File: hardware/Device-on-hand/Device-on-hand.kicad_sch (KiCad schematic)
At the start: 6 parts, among them J1 Conn_01x08, J2 Conn_01x08, J3 Conn_01x02, U1 SparkFun_SEN-14480_H3LIS331DL, U2 ESP32-DEVKIT-V1

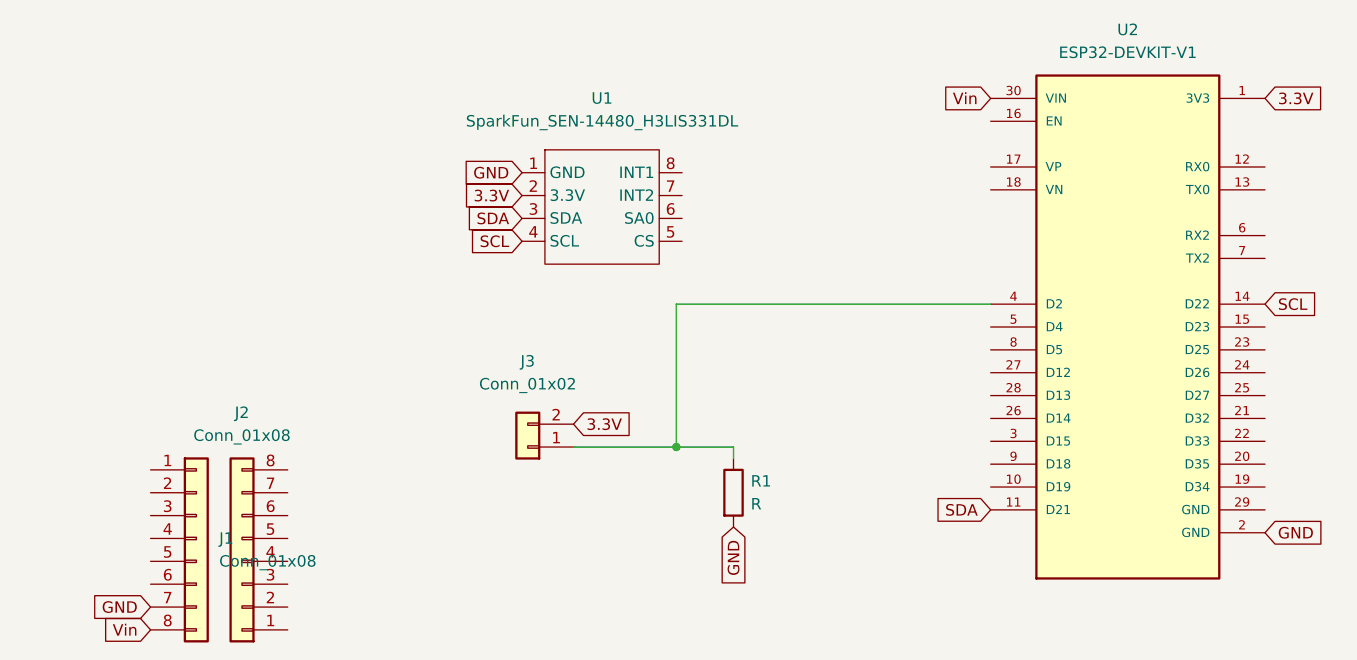
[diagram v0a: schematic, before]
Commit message: update
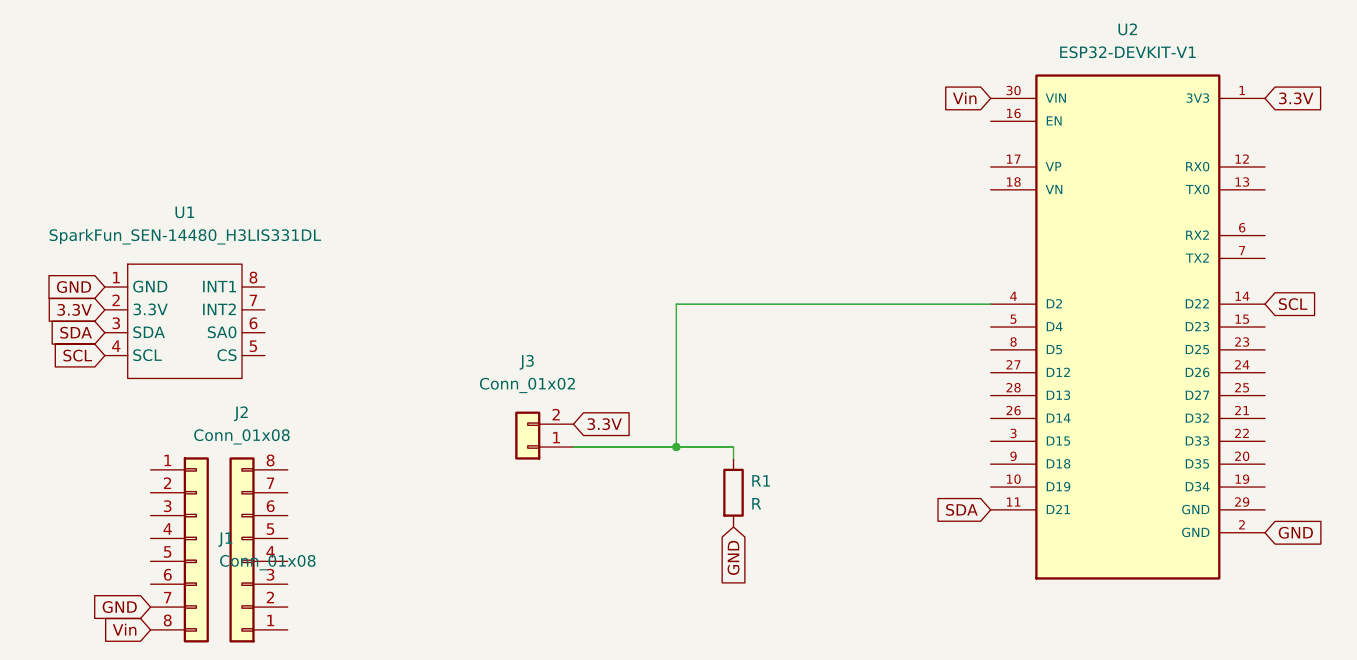
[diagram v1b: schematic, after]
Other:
- moved on the sheet: U1
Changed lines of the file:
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@@
     )
   )
-  (global_label "SCL" (shape input) (at 142.875 84.455 180) (fields_autoplaced)
+  (global_label "SCL" (shape input) (at 96.52 97.155 180) (fields_autoplaced)
     (effects (font (size 1.27 1.27)) (justify right))
-    (property "Intersheet References" "${INTERSHEET_REFS}" (id 0) (at 136.9543 84.3756 0)
+    (property "Intersheet References" "${INTERSHEET_REFS}" (id 0) (at 90.5993 97.0756 0)
       (effects (font (size 1.27 1.27)) (justify right) hide)
     )
@@
     )
   )
-  (global_label "GND" (shape input) (at 142.875 76.835 180) (fields_autoplaced)
+  (global_label "GND" (shape input) (at 96.52 89.535 180) (fields_autoplaced)
     (effects (font (size 1.27 1.27)) (justify right))
-    (property "Intersheet References" "${INTERSHEET_REFS}" (id 0) (at 136.5914 76.7556 0)
+    (property "Intersheet References" "${INTERSHEET_REFS}" (id 0) (at 90.2364 89.4556 0)
       (effects (font (size 1.27 1.27)) (justify right) hide)
     )
@@
     )
   )
-  (global_label "3.3V" (shape input) (at 142.875 79.375 180) (fields_autoplaced)
+  (global_label "3.3V" (shape input) (at 96.52 92.075 180) (fields_autoplaced)
     (effects (font (size 1.27 1.27)) (justify right))
-    (property "Intersheet References" "${INTERSHEET_REFS}" (id 0) (at 136.3495 79.2956 0)
+    (property "Intersheet References" "${INTERSHEET_REFS}" (id 0) (at 89.9945 91.9956 0)
       (effects (font (size 1.27 1.27)) (justify right) hide)
     )
   )
-  (global_label "SDA" (shape input) (at 142.875 81.915 180) (fields_autoplaced)
+  (global_label "SDA" (shape input) (at 96.52 94.615 180) (fields_autoplaced)
     (effects (font (size 1.27 1.27)) (justify right))
-    (property "Intersheet References" "${INTERSHEET_REFS}" (id 0) (at 136.8938 81.8356 0)
+    (property "Intersheet References" "${INTERSHEET_REFS}" (id 0) (at 90.5388 94.5356 0)
       (effects (font (size 1.27 1.27)) (justify right) hide)
     )
@@
     (pin "2")
   )
-  (symbol (lib_id "H3LIS331DL:SparkFun_SEN-14480_H3LIS331DL") (at 151.765 80.645 0) (unit 1)
+  (symbol (lib_id "H3LIS331DL:SparkFun_SEN-14480_H3LIS331DL") (at 105.41 93.345 0) (unit 1)
     (in_bom yes) (on_board yes) (fields_autoplaced)
-    (property "Reference" "U1" (id 0) (at 151.765 68.58 0))
-    (property "Value" "SparkFun_SEN-14480_H3LIS331DL" (id 1) (at 151.765 71.12 0))
-    (property "Footprint" "SparkFun_Tri_Axis_Accel_Breakout-H3LIS331DL:SparkFun_Tri_Axis_Accel_Breakout-H3LIS331DL" (id 2) (at 151.765 80.645 0)
+    (property "Reference" "U1" (id 0) (at 105.41 81.28 0))
+    (property "Value" "SparkFun_SEN-14480_H3LIS331DL" (id 1) (at 105.41 83.82 0))
+    (property "Footprint" "SparkFun_Tri_Axis_Accel_Breakout-H3LIS331DL:SparkFun_Tri_Axis_Accel_Breakout-H3LIS331DL" (id 2) (at 105.41 93.345 0)
       (effects (font (size 1.27 1.27)) hide)
     )
-    (property "Datasheet" "" (id 3) (at 151.765 80.645 0)
+    (property "Datasheet" "" (id 3) (at 105.41 93.345 0)
       (effects (font (size 1.27 1.27)) hide)
     )

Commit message: final commit i hope
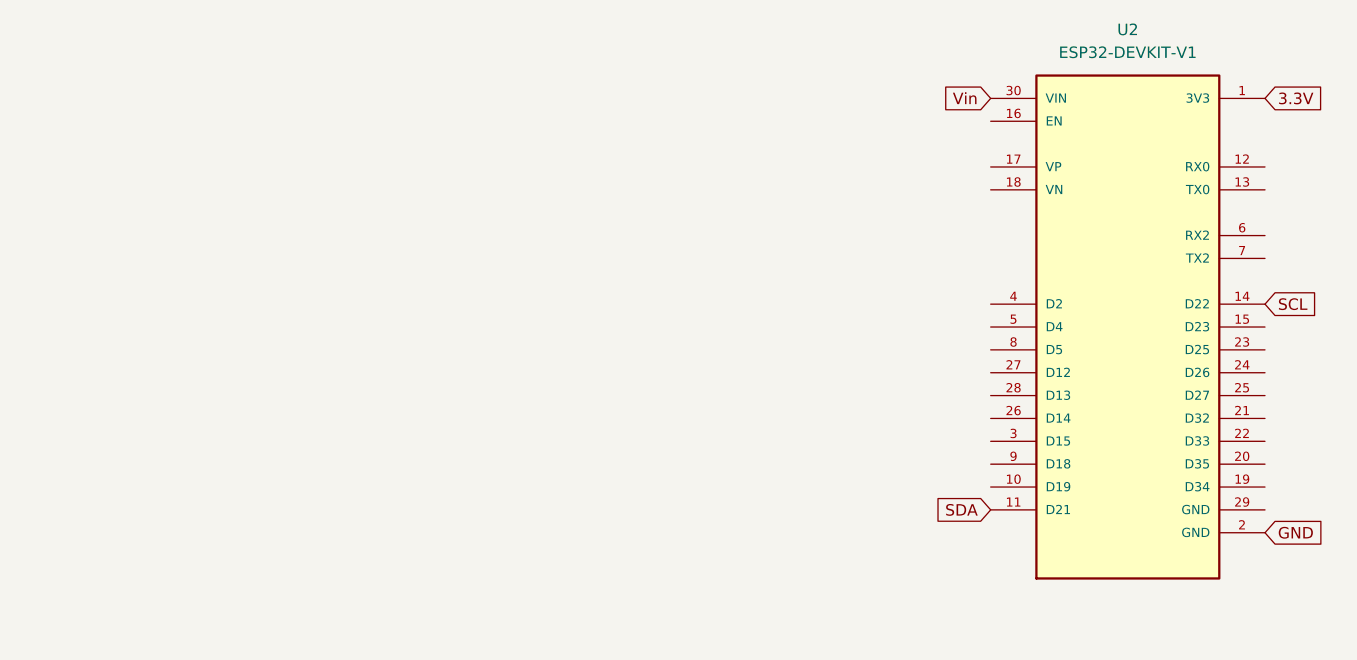
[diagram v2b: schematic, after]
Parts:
- removed J1, J2: Conn_01x08, Connector_PinSocket_2.54mm:PinSocket_1x08_P2.54mm_Vertical, symbol Connector_Generic:Conn_01x08
- removed J3: Conn_01x02, TerminalBlock_Phoenix:TerminalBlock_Phoenix_MKDS-1,5-2-5.08_1x02_P5.08mm_Horizontal, symbol Connector_Generic:Conn_01x02
- removed R1: R, Resistor_THT:R_Axial_DIN0207_L6.3mm_D2.5mm_P10.16mm_Horizontal, symbol Device:R
- removed U1: SparkFun_SEN-14480_H3LIS331DL, SparkFun_Tri_Axis_Accel_Breakout-H3LIS331DL:SparkFun_Tri_Axis_Accel_Breakout-H3LIS331DL, symbol H3LIS331DL:SparkFun_SEN-14480_H3LIS331DL
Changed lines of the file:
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@@
 (kicad_sch (version 20211123) (generator eeschema)
   (paper "A4")
-  (junction (at 160.02 107.315) (diameter 0) (color 0 0 0 0)
-  )
-  (wire (pts (xy 148.59 107.315) (xy 160.02 107.315))
-    (stroke (width 0) (type default) (color 0 0 0 0))
-  )
-  (wire (pts (xy 160.02 91.44) (xy 160.02 107.315))
-    (stroke (width 0) (type default) (color 0 0 0 0))
-  )
-  (wire (pts (xy 166.37 107.315) (xy 166.37 108.585))
-    (stroke (width 0) (type default) (color 0 0 0 0))
-  )
-  (wire (pts (xy 160.02 107.315) (xy 166.37 107.315))
-    (stroke (width 0) (type default) (color 0 0 0 0))
-  )
-  (wire (pts (xy 194.945 91.44) (xy 160.02 91.44))
-    (stroke (width 0) (type default) (color 0 0 0 0))
-  )
-  (global_label "3.3V" (shape input) (at 148.59 104.775 0) (fields_autoplaced)
-    (effects (font (size 1.27 1.27)) (justify left))
-    (property "Intersheet References" "${INTERSHEET_REFS}" (id 0) (at 155.1155 104.8544 0)
-      (effects (font (size 1.27 1.27)) (justify left) hide)
-    )
-  )
   (global_label "SDA" (shape input) (at 194.945 114.3 180) (fields_autoplaced)
     (effects (font (size 1.27 1.27)) (justify right))
     (property "Intersheet References" "${INTERSHEET_REFS}" (id 0) (at 188.9638 114.2206 0)
-      (effects (font (size 1.27 1.27)) (justify right) hide)
-    )
-  )
-  (global_label "SCL" (shape input) (at 96.52 97.155 180) (fields_autoplaced)
-    (effects (font (size 1.27 1.27)) (justify right))
-    (property "Intersheet References" "${INTERSHEET_REFS}" (id 0) (at 90.5993 97.0756 0)
-      (effects (font (size 1.27 1.27)) (justify right) hide)
-    )
-  )
-  (global_label "GND" (shape input) (at 166.37 116.205 270) (fields_autoplaced)
-    (effects (font (size 1.27 1.27)) (justify right))
-    (property "Intersheet References" "${INTERSHEET_REFS}" (id 0) (at 166.2906 122.4886 90)
-      (effects (font (size 1.27 1.27)) (justify right) hide)
-    )
-  )
-  (global_label "GND" (shape input) (at 101.6 125.095 180) (fields_autoplaced)
-    (effects (font (size 1.27 1.27)) (justify right))
-    (property "Intersheet References" "${INTERSHEET_REFS}" (id 0) (at 95.3164 125.0156 0)
-      (effects (font (size 1.27 1.27)) (justify right) hide)
-    )
-  )
-  (global_label "Vin" (shape input) (at 101.6 127.635 180) (fields_autoplaced)
-    (effects (font (size 1.27 1.27)) (justify right))
-    (property "Intersheet References" "${INTERSHEET_REFS}" (id 0) (at 96.3445 127.5556 0)
       (effects (font (size 1.27 1.27)) (justify right) hide)
     )
@@
     (property "Intersheet References" "${INTERSHEET_REFS}" (id 0) (at 231.7086 116.9194 0)
       (effects (font (size 1.27 1.27)) (justify left) hide)
-    )
-  )
-  (global_label "GND" (shape input) (at 96.52 89.535 180) (fields_autoplaced)
-    (effects (font (size 1.27 1.27)) (justify right))
-    (property "Intersheet References" "${INTERSHEET_REFS}" (id 0) (at 90.2364 89.4556 0)
-      (effects (font (size 1.27 1.27)) (justify right) hide)
     )
   )
@@
       (effects (font (size 1.27 1.27)) (justify left) hide)
     )
-  )
-  (global_label "3.3V" (shape input) (at 96.52 92.075 180) (fields_autoplaced)
-    (effects (font (size 1.27 1.27)) (justify right))
-    (property "Intersheet References" "${INTERSHEET_REFS}" (id 0) (at 89.9945 91.9956 0)
-      (effects (font (size 1.27 1.27)) (justify right) hide)
-    )
-  )
-  (global_label "SDA" (shape input) (at 96.52 94.615 180) (fields_autoplaced)
-    (effects (font (size 1.27 1.27)) (justify right))
-    (property "Intersheet References" "${INTERSHEET_REFS}" (id 0) (at 90.5388 94.5356 0)
-      (effects (font (size 1.27 1.27)) (justify right) hide)
-    )
-  )
-  (symbol (lib_id "Device:R") (at 166.37 112.395 0) (unit 1)
-    (in_bom yes) (on_board yes) (fields_autoplaced)
-    (property "Reference" "R1" (id 0) (at 168.275 111.1249 0)
-      (effects (font (size 1.27 1.27)) (justify left))
-    )
-    (property "Value" "R" (id 1) (at 168.275 113.6649 0)
-      (effects (font (size 1.27 1.27)) (justify left))
-    )
-    (property "Footprint" "Resistor_THT:R_Axial_DIN0207_L6.3mm_D2.5mm_P10.16mm_Horizontal" (id 2) (at 164.592 112.395 90)
-      (effects (font (size 1.27 1.27)) hide)
-    )
-    (property "Datasheet" "~" (id 3) (at 166.37 112.395 0)
-      (effects (font (size 1.27 1.27)) hide)
-    )
-    (pin "1")
-    (pin "2")
-  )
-  (symbol (lib_id "H3LIS331DL:SparkFun_SEN-14480_H3LIS331DL") (at 105.41 93.345 0) (unit 1)
-    (in_bom yes) (on_board yes) (fields_autoplaced)
-    (property "Reference" "U1" (id 0) (at 105.41 81.28 0))
-    (property "Value" "SparkFun_SEN-14480_H3LIS331DL" (id 1) (at 105.41 83.82 0))
-    (property "Footprint" "SparkFun_Tri_Axis_Accel_Breakout-H3LIS331DL:SparkFun_Tri_Axis_Accel_Breakout-H3LIS331DL" (id 2) (at 105.41 93.345 0)
-      (effects (font (size 1.27 1.27)) hide)
-    )
-    (property "Datasheet" "" (id 3) (at 105.41 93.345 0)
-      (effects (font (size 1.27 1.27)) hide)
-    )
-    (pin "1")
-    (pin "2")
-    (pin "3")
-    (pin "4")
-    (pin "5")
-    (pin "6")
-    (pin "7")
-    (pin "8")
-  )
-  (symbol (lib_id "Connector_Generic:Conn_01x08") (at 106.68 117.475 0) (unit 1)
-    (in_bom yes) (on_board yes) (fields_autoplaced)
-    (property "Reference" "J1" (id 0) (at 109.22 117.4749 0)
-      (effects (font (size 1.27 1.27)) (justify left))
-    )
-    (property "Value" "Conn_01x08" (id 1) (at 109.22 120.0149 0)
-      (effects (font (size 1.27 1.27)) (justify left))
-    )
-    (property "Footprint" "Connector_PinSocket_2.54mm:PinSocket_1x08_P2.54mm_Vertical" (id 2) (at 106.68 117.475 0)
-      (effects (font (size 1.27 1.27)) hide)
-    )
-    (property "Datasheet" "~" (id 3) (at 106.68 117.475 0)
-      (effects (font (size 1.27 1.27)) hide)
-    )
-    (pin "1")
-    (pin "2")
-    (pin "3")
-    (pin "4")
-    (pin "5")
-    (pin "6")
-    (pin "7")
-    (pin "8")
-  )
-  (symbol (lib_id "Connector_Generic:Conn_01x02") (at 143.51 107.315 180) (unit 1)
-    (in_bom yes) (on_board yes) (fields_autoplaced)
-    (property "Reference" "J3" (id 0) (at 143.51 97.79 0))
-    (property "Value" "Conn_01x02" (id 1) (at 143.51 100.33 0))
-    (property "Footprint" "TerminalBlock_Phoenix:TerminalBlock_Phoenix_MKDS-1,5-2-5.08_1x02_P5.08mm_Horizontal" (id 2) (at 143.51 107.315 0)
-      (effects (font (size 1.27 1.27)) hide)
-    )
-    (property "Datasheet" "~" (id 3) (at 143.51 107.315 0)
-      (effects (font (size 1.27 1.27)) hide)
-    )
-    (pin "1")
-    (pin "2")
-  )
-  (symbol (lib_id "Connector_Generic:Conn_01x08") (at 111.76 120.015 180) (unit 1)
-    (in_bom yes) (on_board yes) (fields_autoplaced)
-    (property "Reference" "J2" (id 0) (at 111.76 103.505 0))
-    (property "Value" "Conn_01x08" (id 1) (at 111.76 106.045 0))
-    (property "Footprint" "Connector_PinSocket_2.54mm:PinSocket_1x08_P2.54mm_Vertical" (id 2) (at 111.76 120.015 0)
-      (effects (font (size 1.27 1.27)) hide)
-    )
-    (property "Datasheet" "~" (id 3) (at 111.76 120.015 0)
-      (effects (font (size 1.27 1.27)) hide)
-    )
-    (pin "1")
-    (pin "2")
-    (pin "3")
-    (pin "4")
-    (pin "5")
-    (pin "6")
-    (pin "7")
-    (pin "8")
   )
   (symbol (lib_id "ESP32-DEVKIT-V1:ESP32-DEVKIT-V1") (at 210.185 93.98 0) (unit 1)
@@
   )
   (symbol_instances
-    (path "/7155b48b-763c-462d-8329-c845182f9e77"
-      (reference "J1") (unit 1) (value "Conn_01x08") (footprint "Connector_PinSocket_2.54mm:PinSocket_1x08_P2.54mm_Vertical")
-    )
-    (path "/e9645483-6666-44ac-be28-8c42b1532b86"
-      (reference "J2") (unit 1) (value "Conn_01x08") (footprint "Connector_PinSocket_2.54mm:PinSocket_1x08_P2.54mm_Vertical")
-    )
-    (path "/999d1759-3613-4b2b-ba58-30384da44b8b"
-      (reference "J3") (unit 1) (value "Conn_01x02") (footprint "TerminalBlock_Phoenix:TerminalBlock_Phoenix_MKDS-1,5-2-5.08_1x02_P5.08mm_Horizontal")
-    )
-    (path "/1cd20397-060e-49ef-aad6-0d34f2a8395a"
-      (reference "R1") (unit 1) (value "R") (footprint "Resistor_THT:R_Axial_DIN0207_L6.3mm_D2.5mm_P10.16mm_Horizontal")
-    )
-    (path "/70750b56-7da4-4217-94ef-dd1a4ff9633b"
-      (reference "U1") (unit 1) (value "SparkFun_SEN-14480_H3LIS331DL") (footprint "SparkFun_Tri_Axis_Accel_Breakout-H3LIS331DL:SparkFun_Tri_Axis_Accel_Breakout-H3LIS331DL")
-    )
     (path "/fe039a15-eb0a-4870-9652-633b741c5c1e"
       (reference "U2") (unit 1) (value "ESP32-DEVKIT-V1") (footprint "ESP32-DEVKIT-V1:MODULE_ESP32_DEVKIT_V1")
